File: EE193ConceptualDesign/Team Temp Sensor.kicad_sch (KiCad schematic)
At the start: 36 parts, among them J1 USB_B_Micro, J2 Battery_Connector, Q1 BC818, Q2 BC818, Q3 BS170F, SW2 SW_DIP_x01, U1 ESP32-C3-WROOM-02, U2 CP2102N-A02-GQFN28, U3 LD1117S33TR_SOT223, U4 MCP9808_MSOP

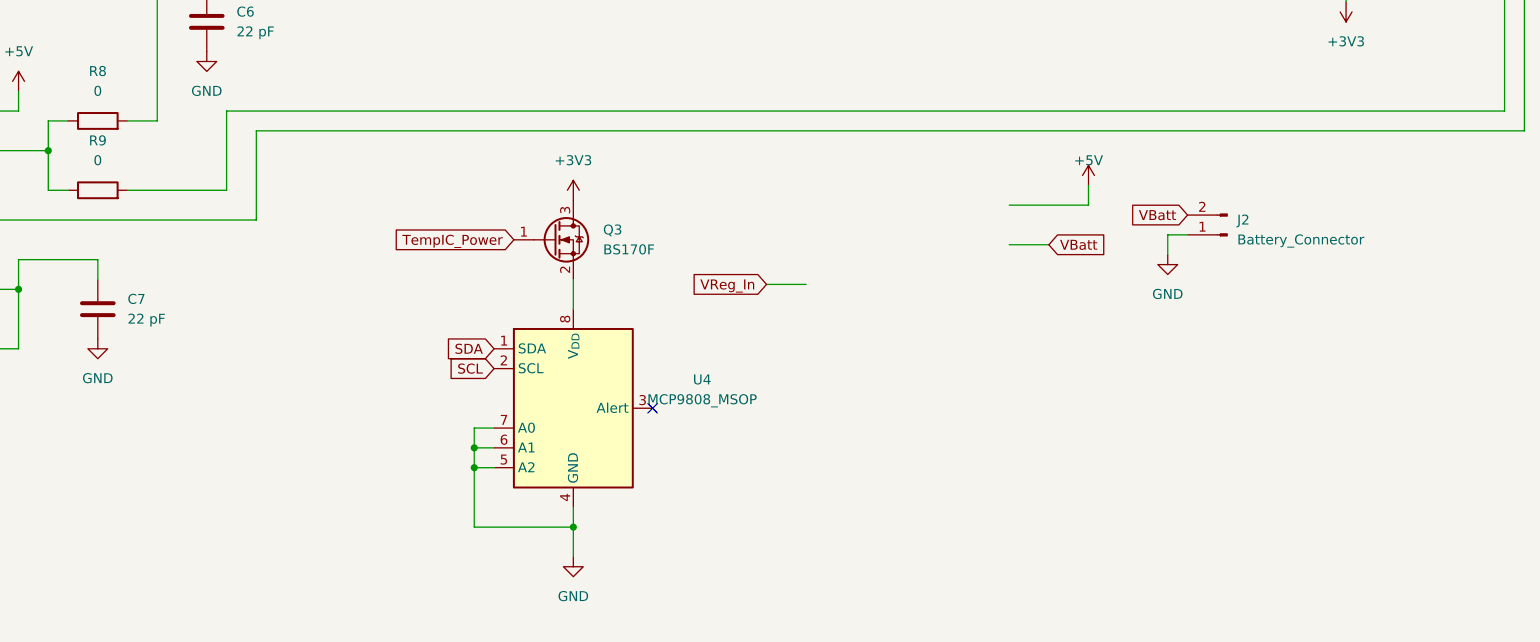
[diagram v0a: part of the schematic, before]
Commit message: v0.3 schematic, layout WIP
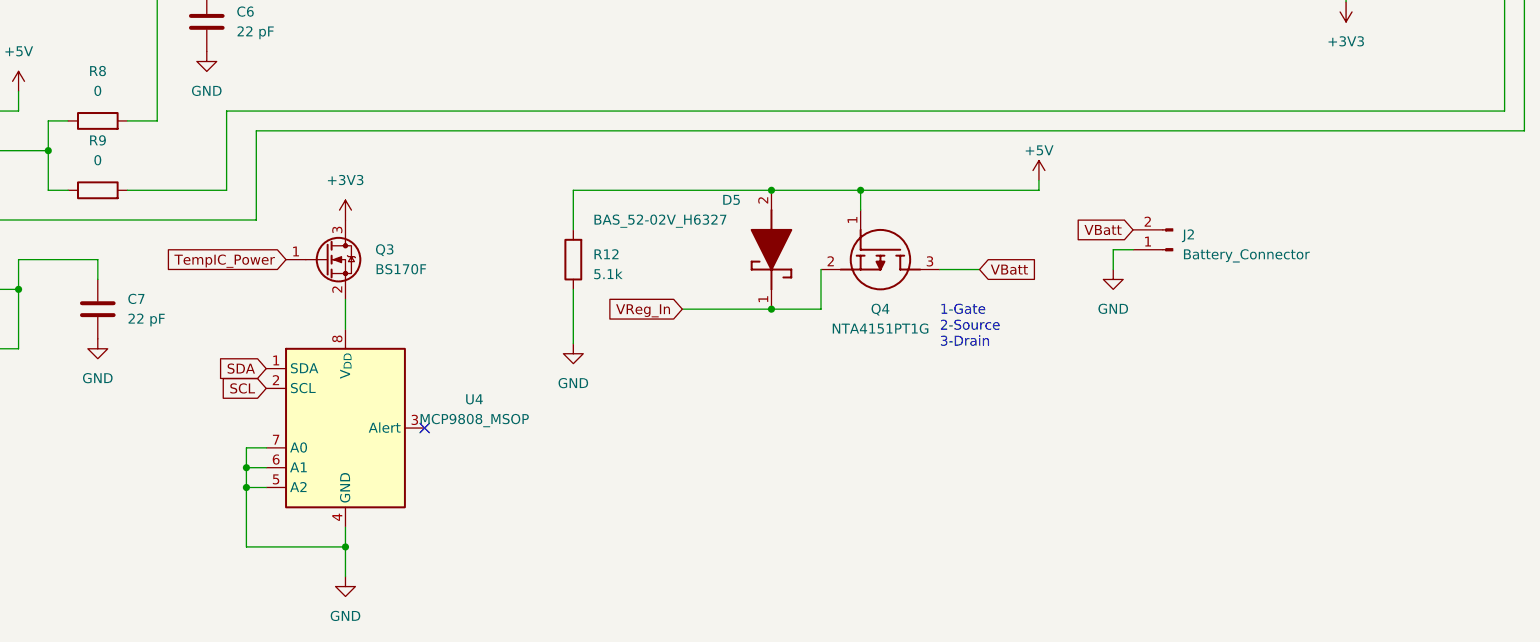
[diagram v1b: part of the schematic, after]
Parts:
- added D5: BAS_52-02V_H6327, SODFL1608X59N, symbol BAS_52-02V_H6327:BAS_52-02V_H6327
- added Q4: NTA4151PT1G, Package_TO_SOT_SMD:SOT-416, symbol NTA4151PT1G:NTA4151PT1G
- added R12: 5.1k, Resistor_SMD:R_0805_2012Metric_Pad1.20x1.40mm_HandSolder, symbol Device:R
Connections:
- net +5V: now also D5.2 (A), Q4.1 (G), R12.2
- net GND: now also R12.1
- net VBatt: now also Q4.3 (D)
- net VReg_In: now also D5.1 (K), Q4.2 (S)
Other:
- note added: "1-Gate 2-Source 3-Drain"
- moved on the sheet: J2, Q3, U4
